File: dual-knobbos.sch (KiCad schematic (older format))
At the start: 34 parts, among them J1 USB_C_Receptacle_USB2.0, SW1 SW_Push, SW2 Rotary_Encoder_Switch, SW3 Rotary_Encoder_Switch, U1 ATmega32U4-AU, Y1 16MHz

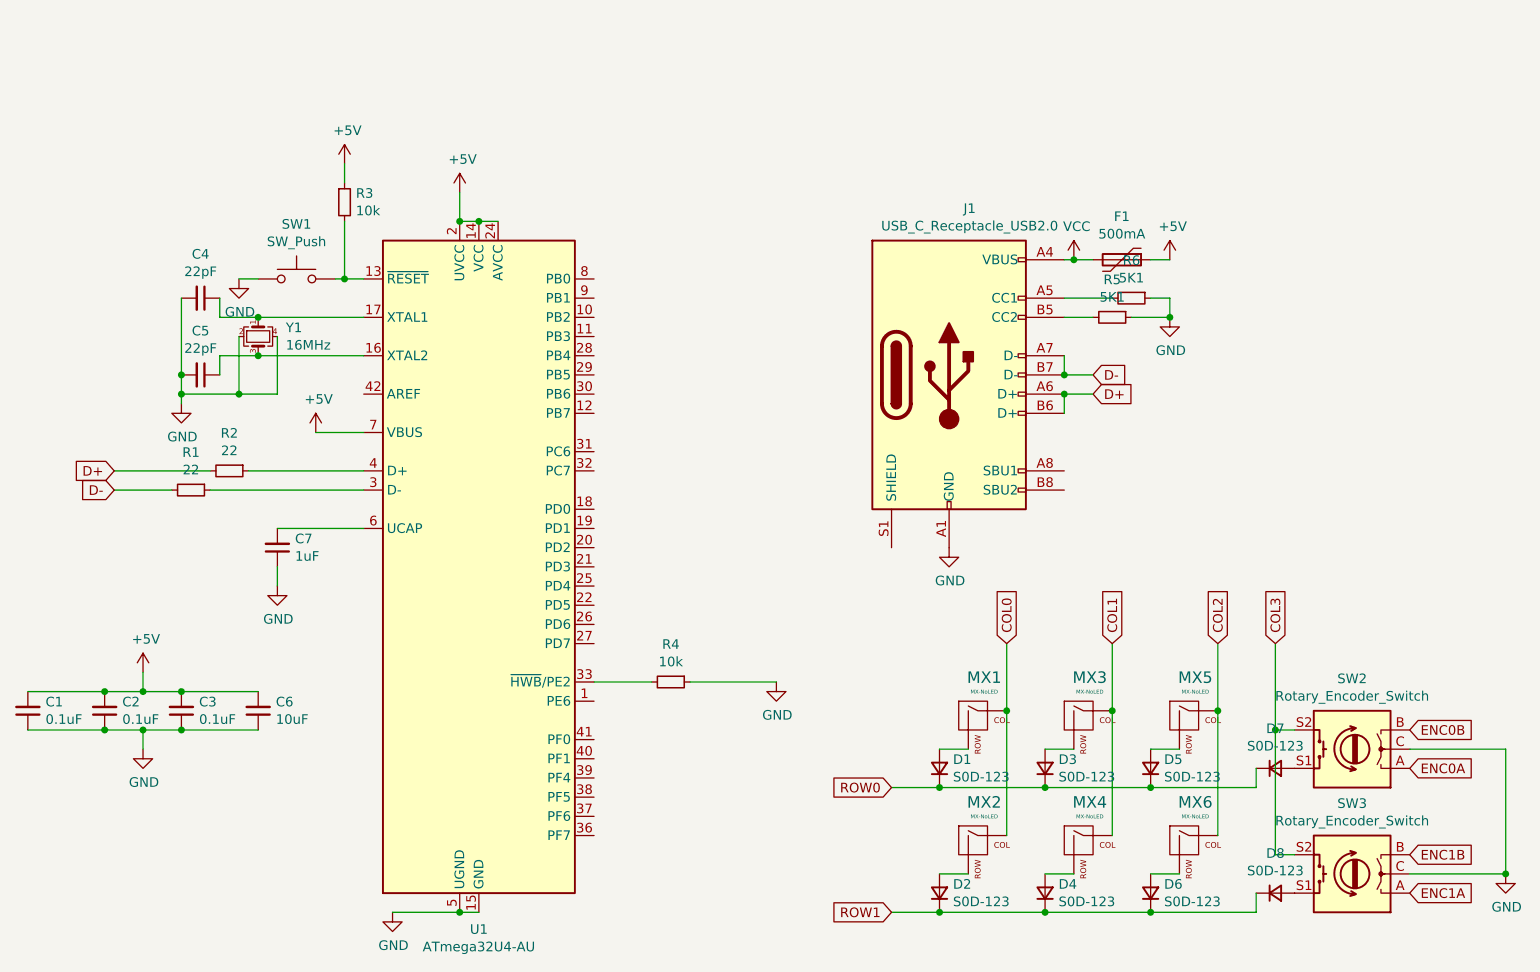
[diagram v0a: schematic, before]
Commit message: mid commit
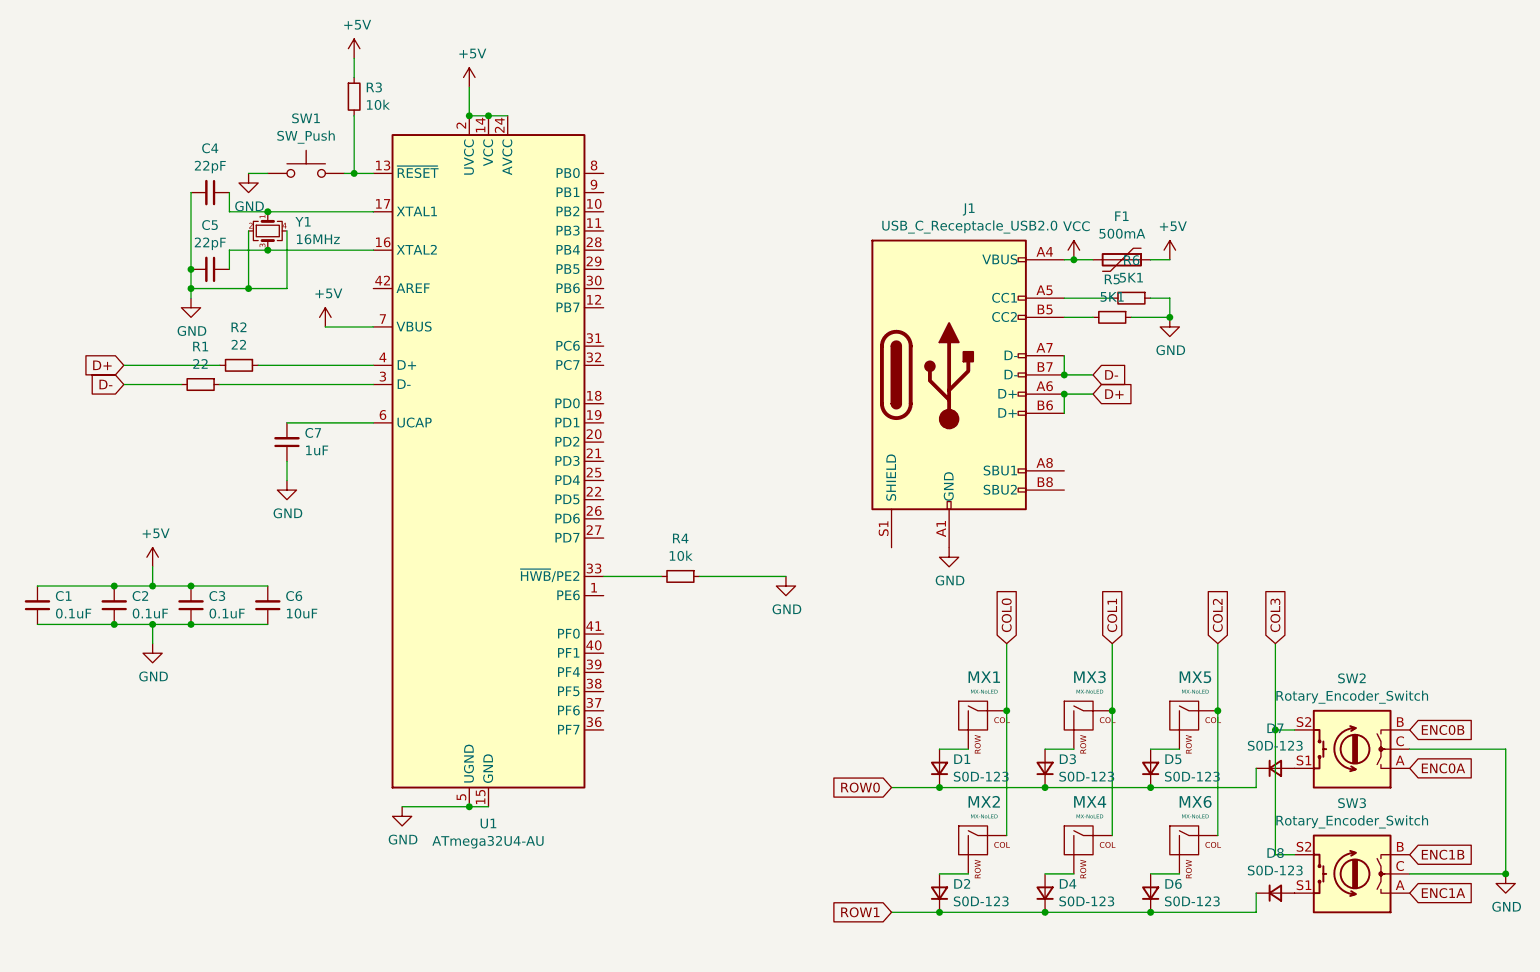
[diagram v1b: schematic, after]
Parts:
- D1, D2, D3, D4, D5, D6, D7, D8: footprint Diode_THT:D_DO-35_SOD27_P2.54mm_Vertical_AnodeUp -> Diode_THT:D_DO-35_SOD27_P5.08mm_Vertical_AnodeUp
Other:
- moved on the sheet: C1, C2, C3, C4, C5, C6, C7, R1, R2, R3, R4, SW1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

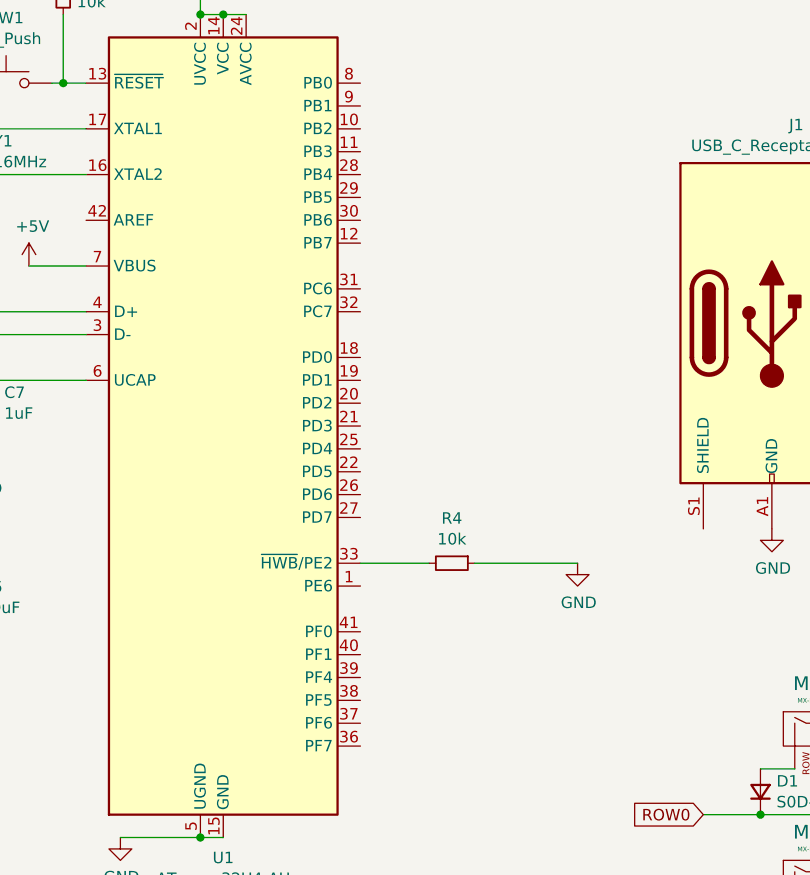
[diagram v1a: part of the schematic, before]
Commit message: some commit idk
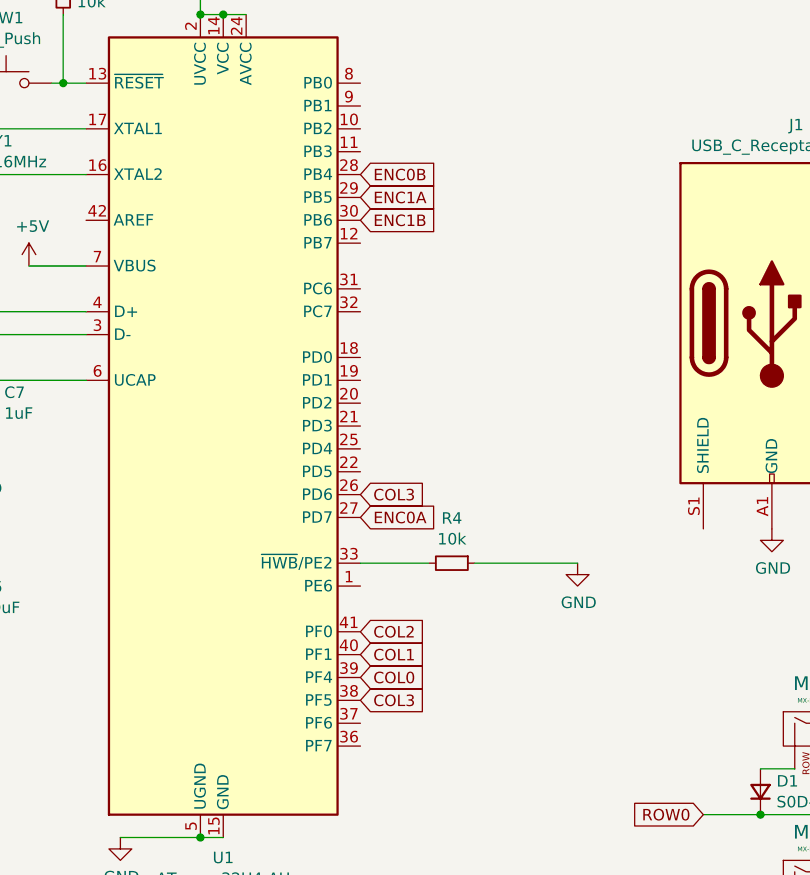
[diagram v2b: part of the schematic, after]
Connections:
- net COL0: now also U1.39 (PF4)
- net COL1: now also U1.40 (PF1)
- net COL2: now also U1.41 (PF0)
- net COL3: now also U1.26 (PD6), U1.38 (PF5)
- net ENC0A: now also U1.27 (PD7)
- net ENC0B: now also U1.28 (PB4)
- net ENC1A: now also U1.29 (PB5)
- net ENC1B: now also U1.30 (PB6)
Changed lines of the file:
@@
 	8750 4650 9250 4650
 Connection ~ 9250 5300
+Text GLabel 4550 3450 2    50   Input ~ 0
+COL3
+Text GLabel 4550 2050 2    50   Input ~ 0
+ENC0B
+Text GLabel 4550 3550 2    50   Input ~ 0
+ENC0A
+Text GLabel 4550 2150 2    50   Input ~ 0
+ENC1A
+Text GLabel 4550 2250 2    50   Input ~ 0
+ENC1B
+Text GLabel 4550 4050 2    50   Input ~ 0
+COL2
+Text GLabel 4550 4150 2    50   Input ~ 0
+COL1
+Text GLabel 4550 4250 2    50   Input ~ 0
+COL0
+Text GLabel 4550 4350 2    50   Input ~ 0
+COL3
 $EndSCHEMATC
